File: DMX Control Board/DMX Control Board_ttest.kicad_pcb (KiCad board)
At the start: 2 copper layers, 136.4 x 91 mm, 32 parts, among them J1 DC_IN, J2 DMX_IN, J3 LED1, J4 LED2, J5 LED3, J6 LED4, U1 ESP32-DevKitC_Headers

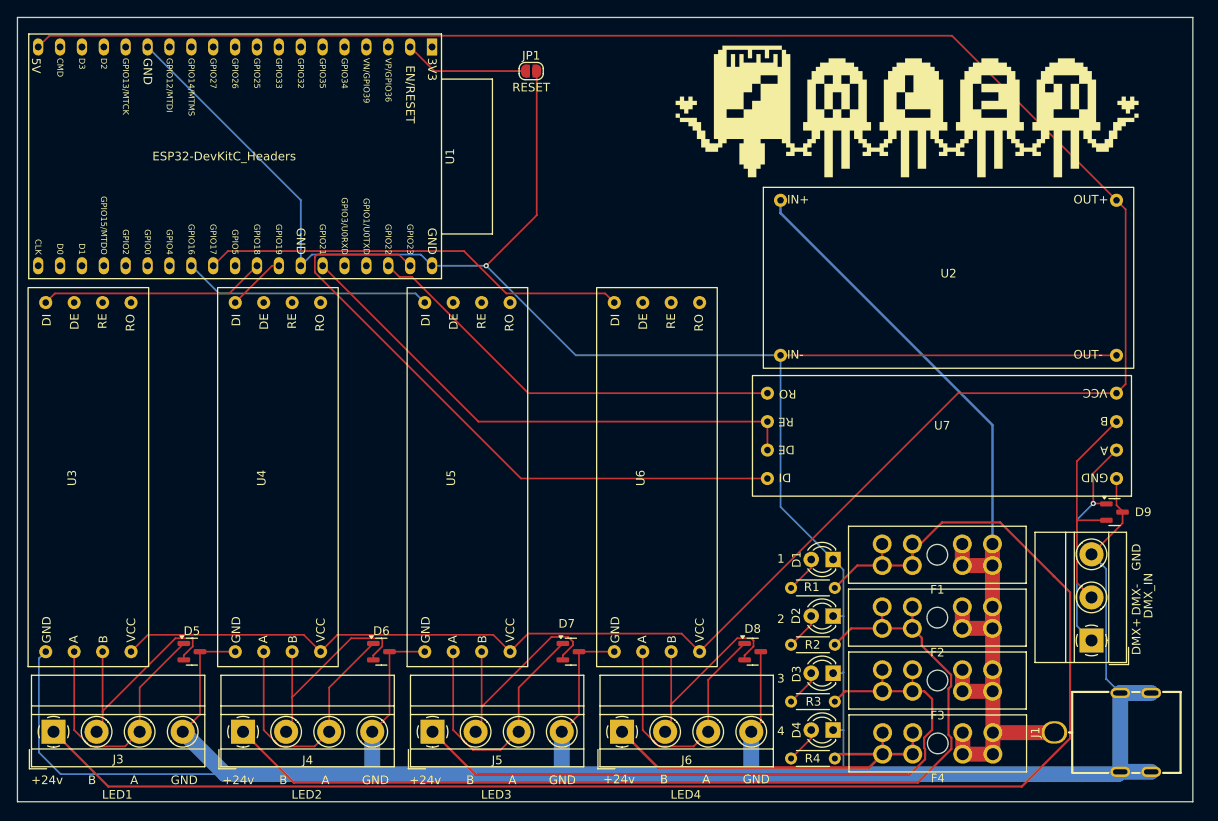
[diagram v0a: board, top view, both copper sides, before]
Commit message: 27th Mega Commit
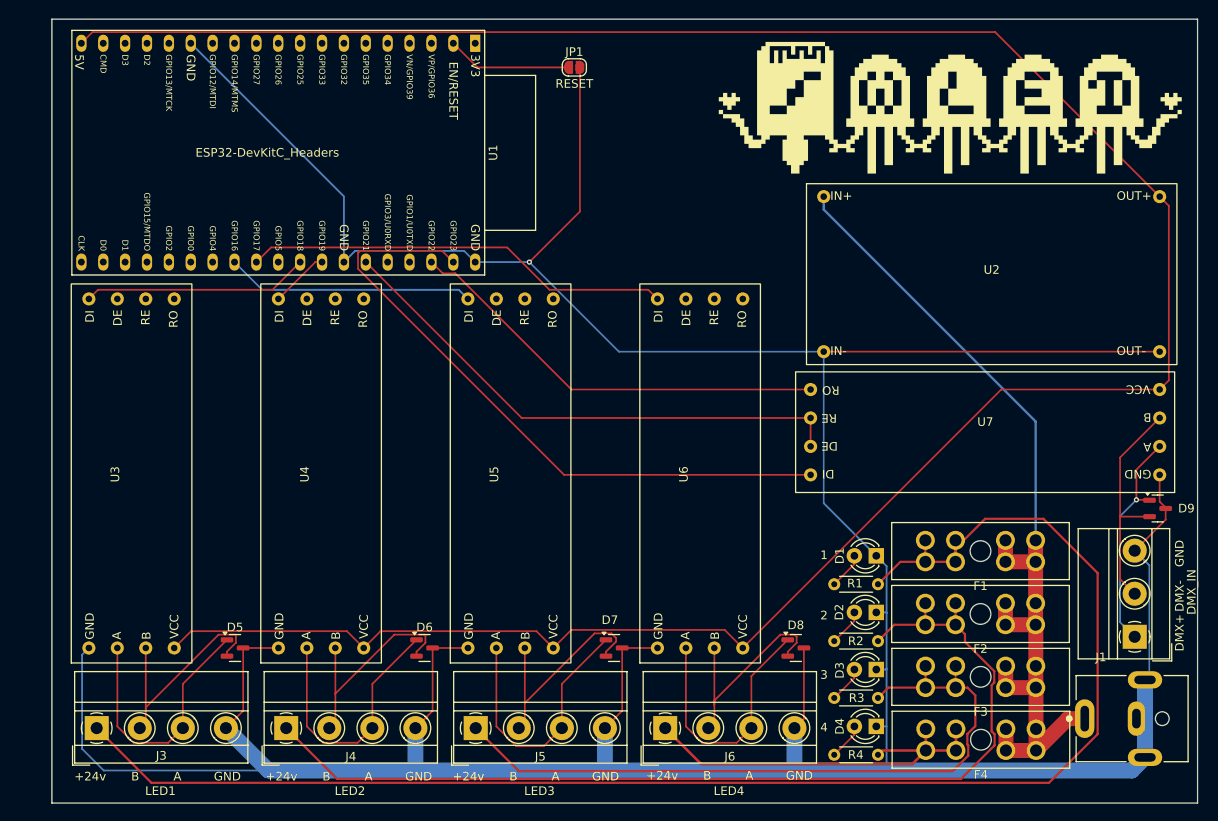
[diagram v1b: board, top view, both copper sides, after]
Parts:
- J1: footprint XUNPU:DC-IN-TH_DC-S010A-D025-20A -> PJ_063AH:CUI_PJ-063AH
- moved F3 5.03 mm to (192.1, 112.6)
- moved R1 5.03 mm to (173.8, 100.6)
- moved U1 5.03 mm to (127.0, 37.8)
- moved U2 5.03 mm to (187.0, 64.6)
- moved U3 5.03 mm to (87.6, 87.8)
- moved U6 5.03 mm to (153.7, 87.8)
- moved F4 5.03 mm to (192.2, 119.9)
- moved JP1 5.03 mm to (138.6, 40.6)
- moved R2 5.03 mm to (173.8, 107.2)
- moved R3 5.03 mm to (173.8, 113.8)
- moved R4 5.03 mm to (173.8, 120.4)
- moved U4 5.03 mm to (109.6, 87.8)
- moved U5 5.03 mm to (131.6, 87.8)
- moved D5 5.03 mm to (99.2, 108.0)
- moved D6 5.03 mm to (121.2, 108.0)
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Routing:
- net GND: track 470.9 -> 464.9 mm
- net Net-(J3-Pin_1): track 179.8 -> 177.0 mm
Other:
- board size 136.4 x 91 mm -> 133 x 91 mm
